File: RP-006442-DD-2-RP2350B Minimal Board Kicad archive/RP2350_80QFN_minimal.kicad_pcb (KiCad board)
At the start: 2 copper layers, 92 x 98 mm, 94 parts, among them J1 USB_C_Receptacle_USB2.0_16P, J2 Conn_02x26_Odd_Even, J3 Conn_02x26_Odd_Even, J4 Conn_01x03, J5 USB_C_Receptacle_USB2.0_16P, SW1 SW_Push, SW2 SW_Push, SW3 SW_Push, SW4 SW_Push, U1 RP2350_80QFN, U2 NCP1117-3.3_SOT223, U3 W25Q128JVS, U4 DNF, U5 W25Q128JVS, U6 NCP1117-3.3_SOT223, U7 RP2350_60QFN, U8 HT16K33A-28SOP, U9 CC56-12EWA, Y1 ABM8-272-T3, Y2 ABM8-272-T3

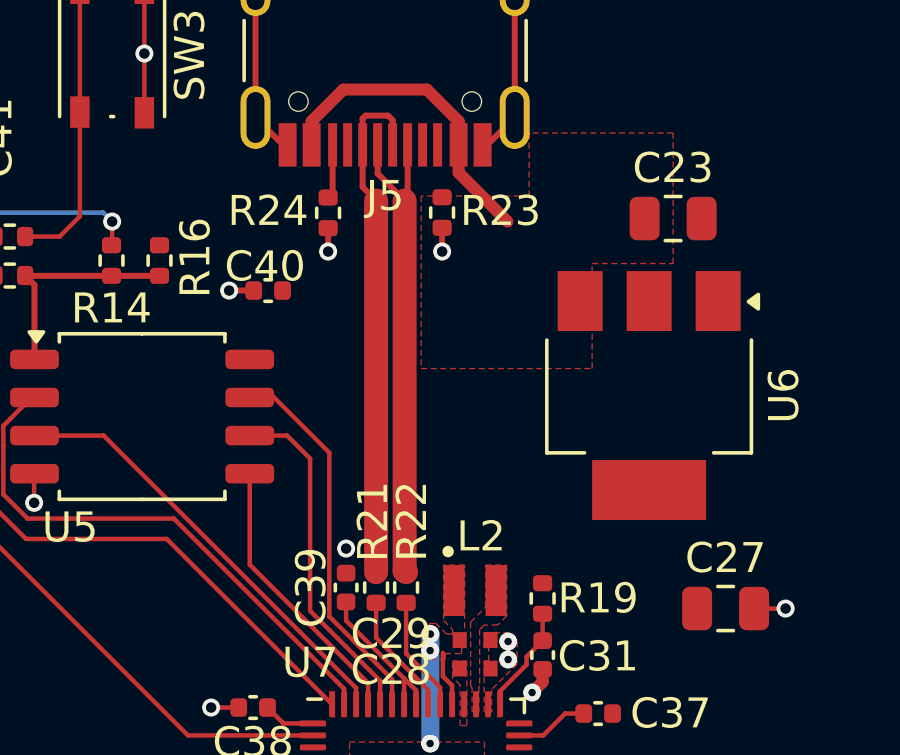
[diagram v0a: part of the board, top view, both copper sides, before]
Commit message: Update to pcb
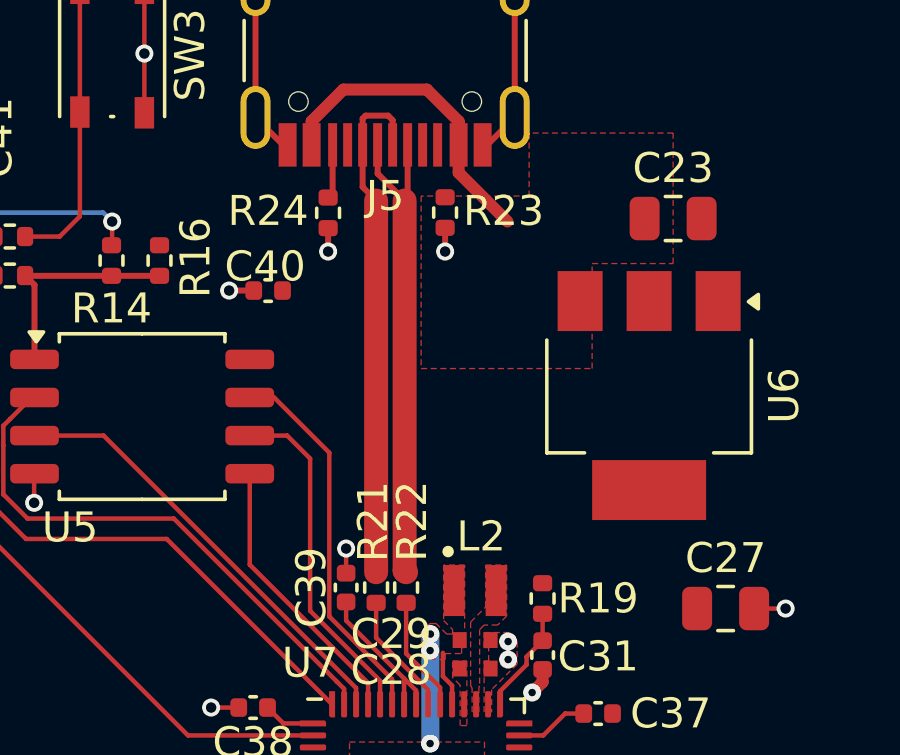
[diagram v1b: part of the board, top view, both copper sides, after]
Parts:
- moved R23 0.10 mm to (147.4, 80.3)
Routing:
- net GND: track 65.8 -> 66.6 mm
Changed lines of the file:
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@@
 	(footprint "Resistor_SMD:R_0402_1005Metric"
 		(layer "F.Cu")
-		(at 147.3 80.3 90)
+		(at 147.4 80.3 90)
 		(descr "Resistor SMD 0402 (1005 Metric), square (rectangular) end terminal, IPC_7351 nominal, (Body size source: IPC-SM-782 page 72, https://www.pcb-3d.com/wordpress/wp-content/uploads/ipc-sm-782a_amendment_1_and_2.pdf), generated with kicad-footprint-generator")
 		(tags "resistor")
@@
 	)
 	(segment
+		(start 144.1 92.32)
+		(end 144.1 91.5)
+		(width 0.15)
+		(layer "F.Cu")
+		(net 1)
+	)
+	(segment
 		(start 108.8875 78.75)
 		(end 109.8875 79.75)
@@
 	)
 	(segment
-		(start 147.3 80.81)
-		(end 147.3 81.6)
+		(start 147.4 80.81)
+		(end 147.4 81.6)
 		(width 0.2)
 		(layer "F.Cu")
@@
 	)
 	(via
-		(at 147.3 81.6)
+		(at 147.4 81.6)
 		(size 0.6)
 		(drill 0.35)
@@
 	)
 	(zone
+		(net 0)
+		(net_name "")
+		(layer "F.Cu")
+		(hatch edge 0.508)
+		(connect_pads
+			(clearance 0)
+		)
+		(min_thickness 0.2)
+		(filled_areas_thickness no)
+		(keepout
+			(tracks allowed)
+			(vias allowed)
+			(pads allowed)
+			(copperpour not_allowed)
+			(footprints allowed)
+		)
+		(placement
+			(enabled no)
+			(sheetname "/")
+		)
+		(fill
+			(thermal_gap 0.3)
+			(thermal_bridge_width 0.3)
+		)
+		(polygon
+			(pts
+				(xy 143.7 88.2) (xy 144.5 88.2) (xy 144.5 91.2) (xy 143.7 91.2)
+			)
+		)
+	)
+	(zone
 		(net 6)
 		(net_name "+1V1")
@@
 		(layer "F.Cu")
 		(hatch edge 0.508)
-		(priority 10)
+		(priority 20)
 		(connect_pads
 			(clearance 0.2)
@@
 		(net_name "")
 		(layer "F.Cu")
+		(hatch edge 0.508)
+		(connect_pads
+			(clearance 0)
+		)
+		(min_thickness 0.15)
+		(filled_areas_thickness no)
+		(keepout
+			(tracks allowed)
+			(vias allowed)
+			(pads allowed)
+			(copperpour not_allowed)
+			(footprints allowed)
+		)
+		(placement
+			(enabled no)
+			(sheetname "")
+		)
+		(fill
+			(thermal_gap 0.3)
+			(thermal_bridge_width 0.3)
+		)
+		(polygon
+			(pts
+				(xy 133.5 85.2) (xy 133.5 90) (xy 138.6 90) (xy 143.3 94.7) (xy 145.1 94.7) (xy 145.1 92.083333)
+				(xy 141.4 89) (xy 141.4 85.2)
+			)
+		)
+	)
+	(zone
+		(net 0)
+		(net_name "")
+		(layer "F.Cu")
 		(hatch edge 0.5)
 		(connect_pads
@@
 			)
 		)
+	)
+	(zone
+		(net 0)
+		(net_name "")
+		(layer "F.Cu")
+		(hatch edge 0.508)
+		(connect_pads
+			(clearance 0)
+		)
+		(min_thickness 0.15)
+		(filled_areas_thickness no)
+		(keepout
+			(tracks allowed)
+			(vias allowed)
+			(pads allowed)
+			(copperpour not_allowed)
+			(footprints allowed)
+		)
+		(placement
+			(enabled no)
+			(sheetname "")
+		)
+		(fill
+			(thermal_gap 0.3)
+			(thermal_bridge_width 0.3)
+		)
+		(polygon
+			(pts
+				(xy 144.8125 79.15) (xy 146.9 79.15) (xy 146.9 90.2) (xy 146.9 88.4) (xy 146.9 91.4) (xy 144.1 91.4)
+				(xy 144.1 78.9)
+			)
+		)

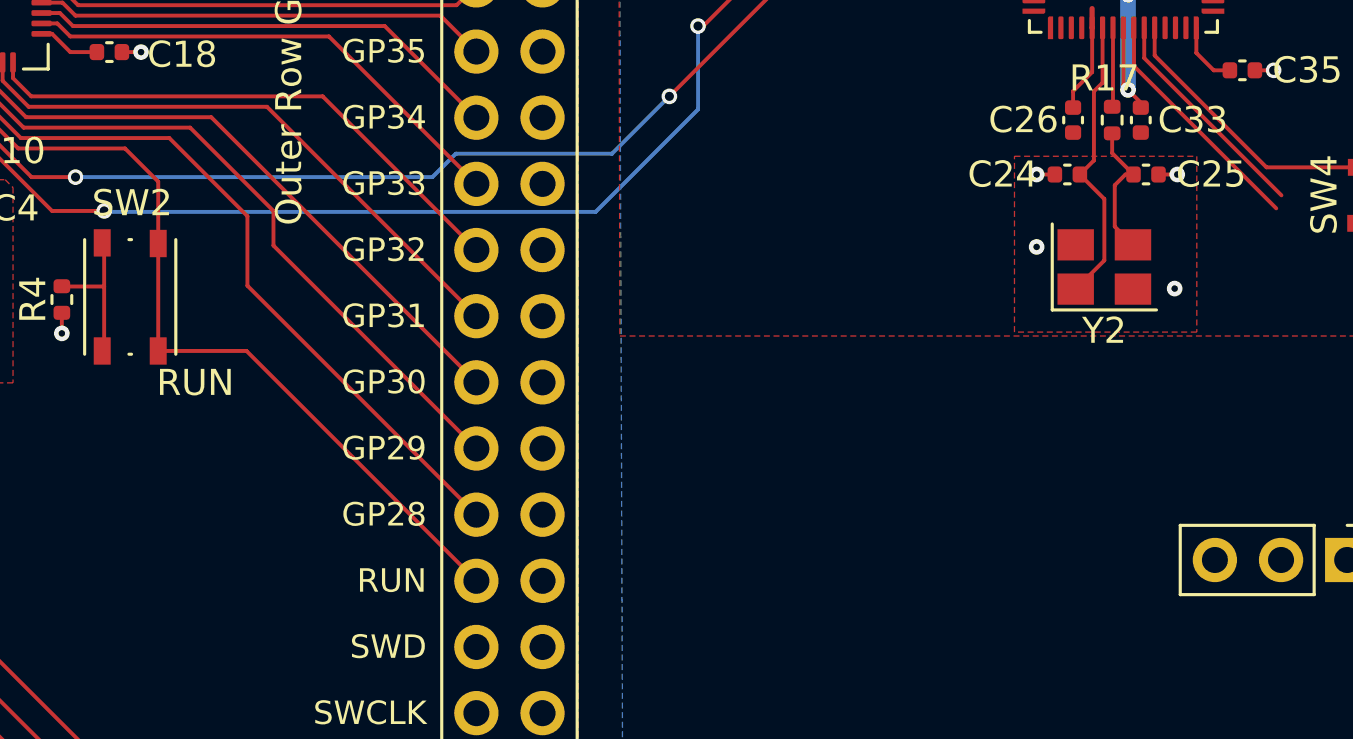
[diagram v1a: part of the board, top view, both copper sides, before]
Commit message: Update to pcb
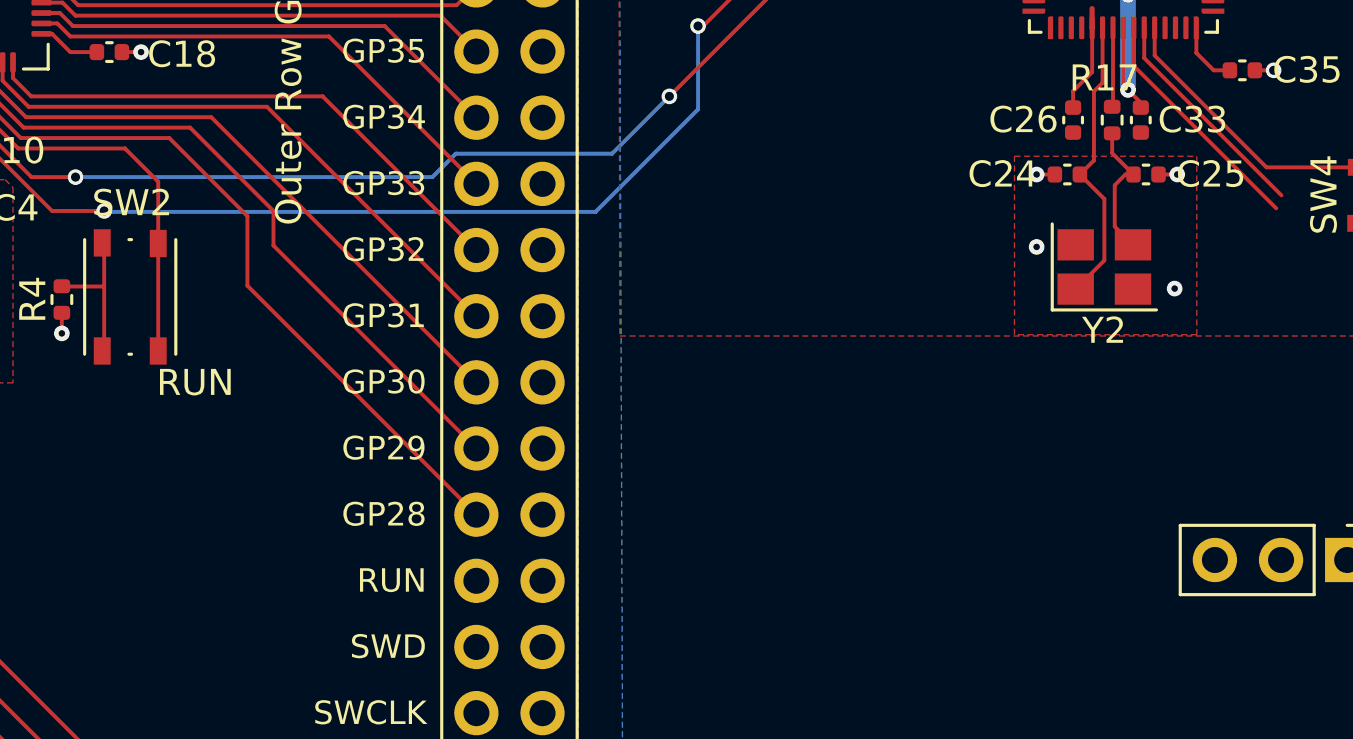
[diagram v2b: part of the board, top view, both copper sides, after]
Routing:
- net /RUN: track 32.5 -> 16.6 mm
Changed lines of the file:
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@@
 	)
 	(segment
-		(start 112.765 115.975)
-		(end 121.59 124.8)
-		(width 0.15)
-		(layer "F.Cu")
-		(net 34)
-	)
-	(segment
 		(start 109.375 115.975)
 		(end 109.375 111.85)
@@
 	)
 	(segment
-		(start 109.375 115.975)
-		(end 112.765 115.975)
-		(width 0.15)
-		(layer "F.Cu")
-		(net 34)
-	)
-	(segment
 		(start 101.8 104.8965)
 		(end 101.8 106)
@@
 		(polygon
 			(pts
-				(xy 142.25 108.5) (xy 149.25 108.5) (xy 149.25 115.25) (xy 142.25 115.25)
+				(xy 142.25 108.5) (xy 149.25 108.5) (xy 149.25 115.35) (xy 142.25 115.35)
 			)
 		)
@@
 		(polygon
 			(pts
-				(xy 145.3 103.7) (xy 145.3 108.1) (xy 141.8 108.1) (xy 141.8 105) (xy 143.1 103.7)
+				(xy 145.3 103.7) (xy 145.3 108.5) (xy 141.8 108.5) (xy 141.8 105) (xy 143.1 103.7)
 			)
 		)
